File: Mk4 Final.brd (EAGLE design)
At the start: 121.6 x 82.5 mm, 310 parts, among them IC1 MSP432E401, IC10 TPD3E001DRL, IC11 TLV9002IDGK, IC12 SN74HC4066D, IC13 TPA2006D1, IC14 MX25R1635FM1IL0, IC15 CC3120R, IC16 TMP102, IC17 OPT3001, IC18 DRV5055, IC2 AS4C4M16SA-7TCN, IC3 HDC2080, IC4 TCA9555RGER, IC5 SIM800C24 S2-10686-Z1L09, IC6 MX25R8035FM1IH1, IC7 TPD3E001DRL, IC8 BQ25601, IC9 TPS62822DLCR, J1 78723-1001, J10 H4P-SMD-2.0, J2 ER-CON50HT-1, J3 2x5 1.27mm, J4 GSM-COIL-ANT, J5 S2B-PH-SM4-TB(LF)(SN), J8 H4P-SMD-2.0, J9 PJ-393-A, Q1 2N7002PW, Q2 2N7002PW, Q3 CSD25402Q3A, Q8 CSD13202Q2, SW1 JOYSTICK, U1 ZX62-B-5PA(33), U4 MIC-6MM, U5 LDMS1540S-01-R8-0.8-R, X1 ABS07-32.768KHZ-T, X2 ABM8G-25.000MHZ-B4Y-T, X3 ABS07-32.768KHZ-T, X4 ABM8-40.000MHZ-10-1-U-T

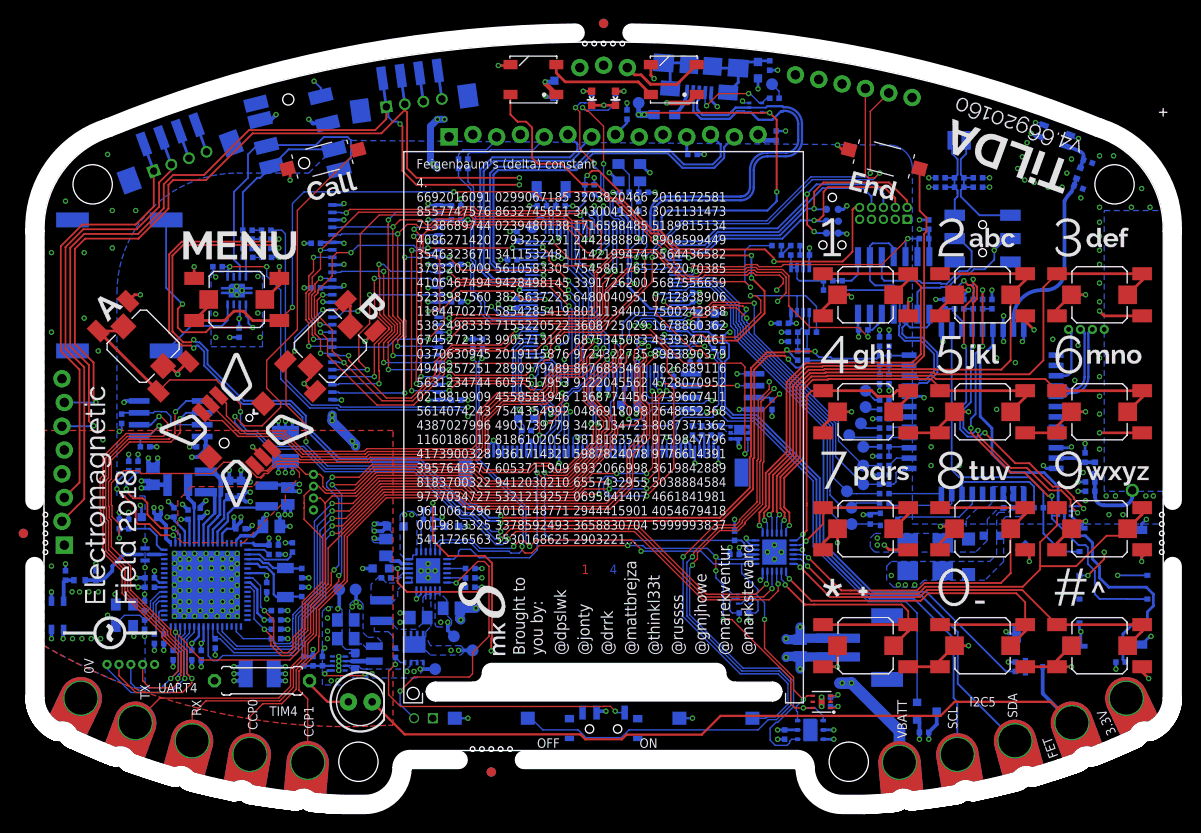
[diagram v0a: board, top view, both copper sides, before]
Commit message: Final design before panel
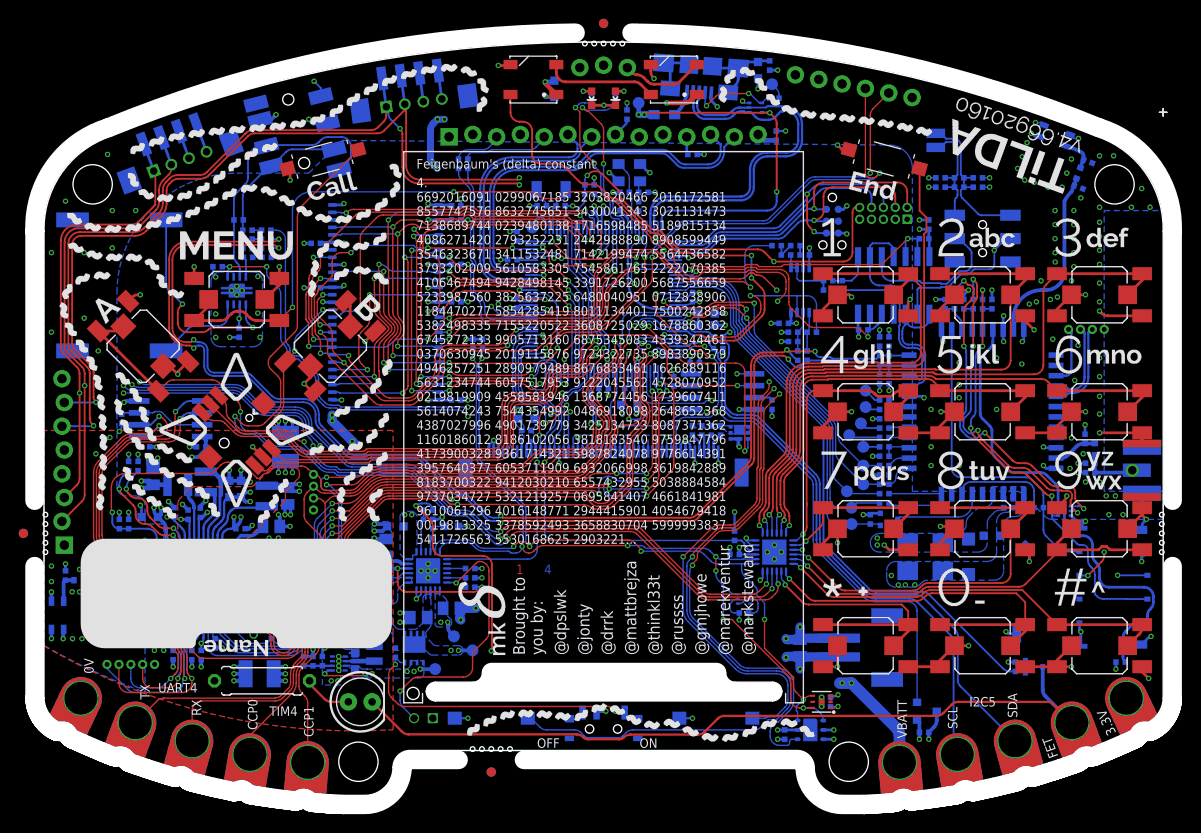
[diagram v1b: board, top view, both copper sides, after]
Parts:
- added ARTWORK5: ARTWORK_NAME_BLOCK, TiLDA Mk4 Parts:TILAD_ARTWORK_NAME
- added ARTWORK6: ARTWORK_MK4-JAKE, TiLDA Mk4 Parts:TILDA_ARTWORK_JAKE
- added J7: SMA-142-0711-821/826, CISECO eaglecad designs:J502-ND-142-0711-821/826-LWK1
- added LOGO5: EMFLOGO-2018-6MM, TiLDA Mk4 Parts:EMFLOGO-2018-6MM
- added R75: 0402/0R/5%, TiLDA Mk4 Parts:R0402-SMALLER
- added TP19: TP, TiLDA Mk4 Parts:P1-06-OCT-CAN
- moved LOGO2 41.3 mm to (3.75, 21.7)
- moved LAYERS1 7.00 mm to (-9.50, 23.5)
- moved U4 2.50 mm to (35.5, 70.0), turned to 270 degrees
- moved J4 2.15 mm to (56.5, 34.8)
- moved C72 2.00 mm to (51.5, 38.1)
- moved C73 2.00 mm to (52.0, 35.5)
- moved D2 2.00 mm to (52.0, 34.5)
- moved L3 2.00 mm to (52.5, 37.0)
- turned S9 to 180 degrees
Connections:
- new net CC_TEST62: IC15.62, TP19.TP
- net AMP_IN_P: now also R75.2
- net AMP_IN_TRS_P: now also R75.1
- net GMS_ANT_L: now also J7.1
- net GND: now also J7.G@1, J7.G@2, J7.G@3, J7.G@4
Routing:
- net UART4_EXT_RX: track 163.9 -> 156.6 mm, vias 3 -> 6
- net BTN_9: track 50.7 -> 43.8 mm
- net CC_!RESET: track 90.5 -> 84.8 mm
- net T4CCP1: track 134.6 -> 129.4 mm, vias 1 -> 3
- net !WAKE: track 121.1 -> 117.7 mm
- net UART3_CC_TX: track 83.5 -> 80.4 mm
- net CC_TEST62: track 0.00 -> 3.11 mm
- net MIC_MUX_P: track 17.5 -> 14.6 mm
- net SSI2_CC_!CS: track 78.1 -> 75.2 mm
- net UART3_CC_RX: track 88.3 -> 85.4 mm
- net SPK_N: track 129.0 -> 126.2 mm
- net SPK_P: track 128.8 -> 126.0 mm
- net MIC_MUX_N: track 25.5 -> 22.9 mm
- net T4CCP0: track 128.5 -> 131.0 mm, vias 1 -> 3
- net SSI2_CC_MOSI: track 79.2 -> 76.7 mm
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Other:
- board text added: "T62"
- board text added: "badge.emfcamp.org/2018"
- board text added: "designed and assembled in the UK"
